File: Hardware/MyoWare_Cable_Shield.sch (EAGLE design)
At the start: 13 parts

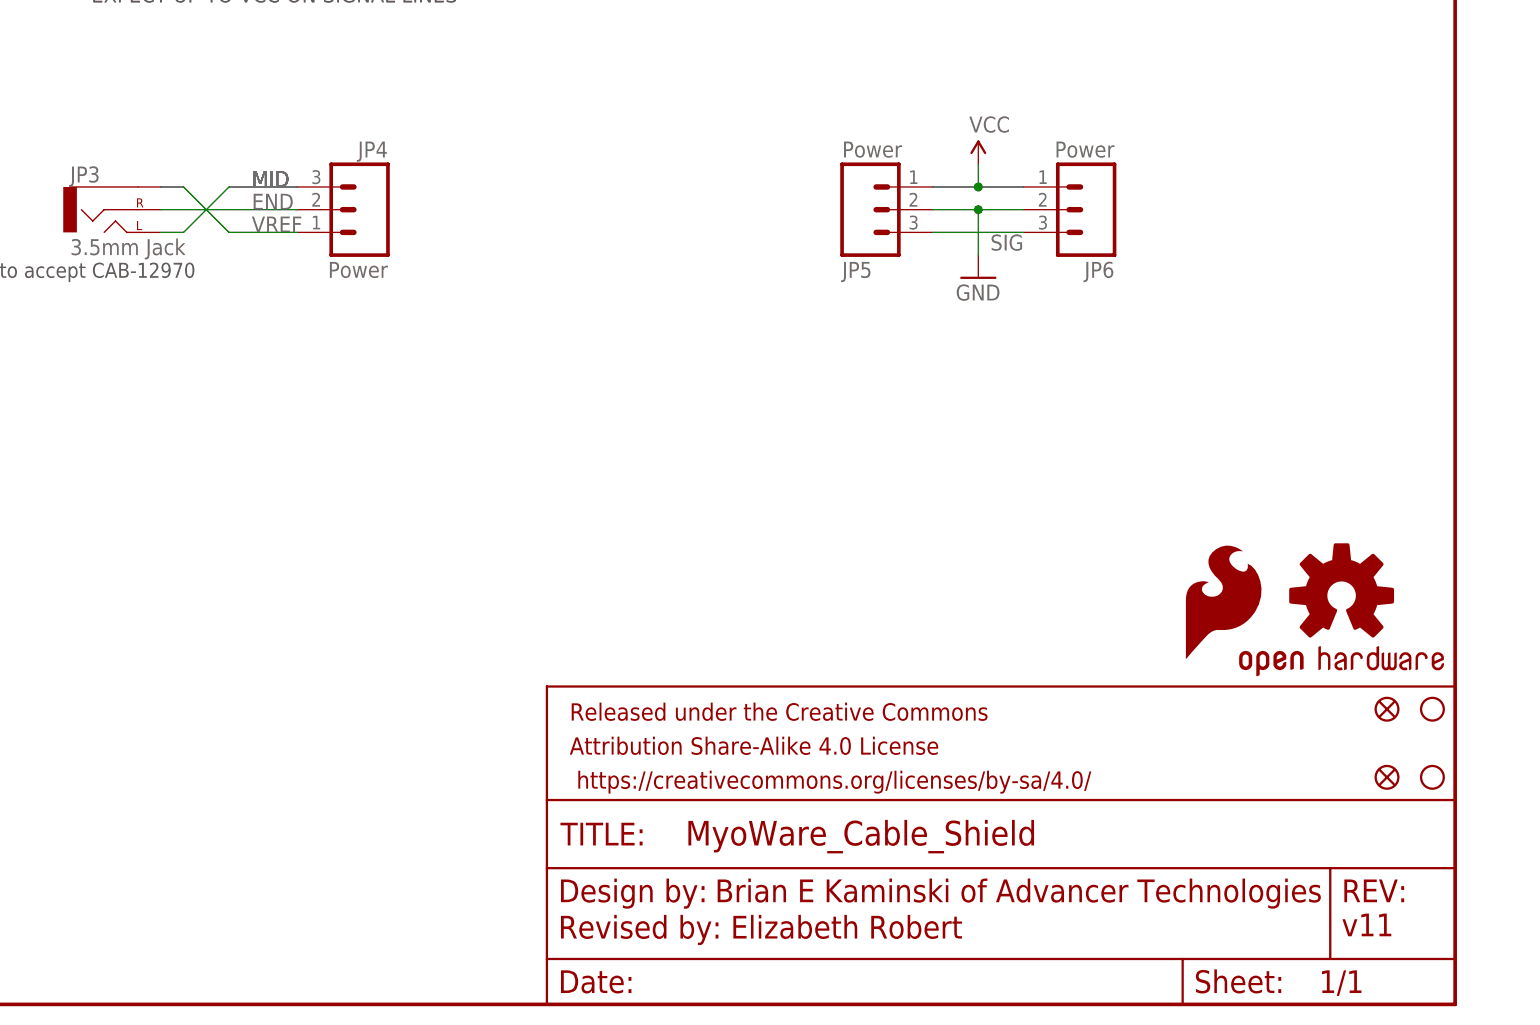
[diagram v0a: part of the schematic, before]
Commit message: Revert "V11"
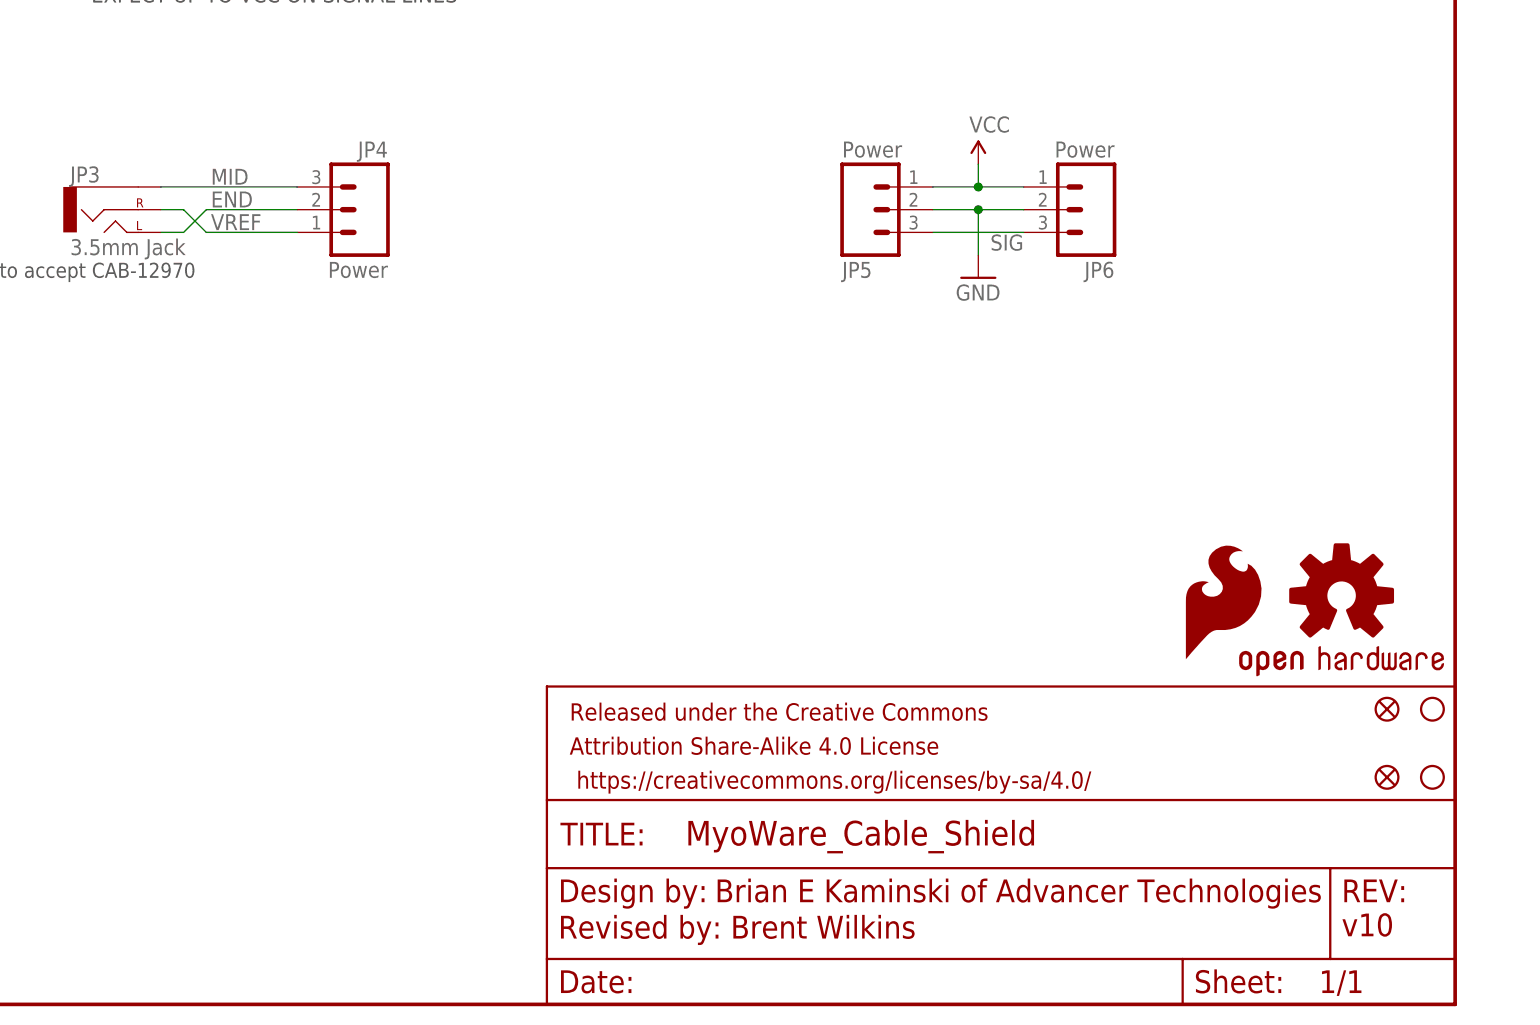
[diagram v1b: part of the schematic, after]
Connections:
- net END: now also JP3.LEFT; no longer JP3.RIGHT
- net MID: now also JP3.SLEEVE; no longer JP3.LEFT
- net VREF: now also JP3.RIGHT; no longer JP3.SLEEVE
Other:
- note added: "Revised by: Brent Wilkins"
- note added: "v10"
- note removed: "Revised by: Elizabeth Robert"
- note removed: "v11"
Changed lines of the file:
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@@
 <?xml version="1.0" encoding="utf-8"?>
 <!DOCTYPE eagle SYSTEM "eagle.dtd">
-<eagle version="7.7.0">
+<eagle version="7.4.0">
 <drawing>
 <settings>
@@
 <plain>
 <text x="166.116" y="11.43" size="2.54" layer="94">Brian E Kaminski of Advancer Technologies</text>
-<text x="148.59" y="7.366" size="2.54" layer="94" ratio="10">Revised by: Elizabeth Robert</text>
-<text x="236.22" y="7.62" size="2.54" layer="94" font="vector">v11</text>
+<text x="148.59" y="7.366" size="2.54" layer="94" ratio="10">Revised by: Brent Wilkins</text>
+<text x="236.22" y="7.62" size="2.54" layer="94" font="vector">v10</text>
 <text x="116.84" y="114.3" size="1.778" layer="97" font="vector" ratio="15" align="center">VCC (+VS) +2.7V to +5.9V
 EXPECT UP TO VCC ON SIGNAL LINES</text>
@@
 </busses>
 <nets>
+<net name="MID" class="0">
+<segment>
+<pinref part="JP4" gate="G$1" pin="3"/>
+<label x="109.728" y="91.694" size="1.778" layer="95"/>
+<wire x1="104.14" y1="91.44" x2="119.38" y2="91.44" width="0.1524" layer="91"/>
+<pinref part="JP3" gate="G$1" pin="SLEEVE"/>
+</segment>
+</net>
+<net name="END" class="0">
+<segment>
+<pinref part="JP4" gate="G$1" pin="2"/>
+<label x="109.728" y="89.154" size="1.778" layer="95"/>
+<wire x1="109.22" y1="88.9" x2="119.38" y2="88.9" width="0.1524" layer="91"/>
+<pinref part="JP3" gate="G$1" pin="LEFT"/>
+<wire x1="104.14" y1="86.36" x2="106.68" y2="86.36" width="0.1524" layer="91"/>
+<wire x1="106.68" y1="86.36" x2="109.22" y2="88.9" width="0.1524" layer="91"/>
+</segment>
+</net>
+<net name="VREF" class="0">
+<segment>
+<pinref part="JP4" gate="G$1" pin="1"/>
+<label x="109.728" y="86.614" size="1.778" layer="95"/>
+<wire x1="109.22" y1="86.36" x2="119.38" y2="86.36" width="0.1524" layer="91"/>
+<pinref part="JP3" gate="G$1" pin="RIGHT"/>
+<wire x1="104.14" y1="88.9" x2="106.68" y2="88.9" width="0.1524" layer="91"/>
+<wire x1="106.68" y1="88.9" x2="109.22" y2="86.36" width="0.1524" layer="91"/>
+</segment>
+</net>
 <net name="SHIELD" class="0">
 <segment>
@@
 </segment>
 </net>
-<net name="MID" class="0">
-<segment>
-<pinref part="JP4" gate="G$1" pin="3"/>
-<wire x1="119.38" y1="91.44" x2="111.76" y2="91.44" width="0.1524" layer="91"/>
-<wire x1="111.76" y1="91.44" x2="106.68" y2="86.36" width="0.1524" layer="91"/>
-<pinref part="JP3" gate="G$1" pin="LEFT"/>
-<wire x1="106.68" y1="86.36" x2="104.14" y2="86.36" width="0.1524" layer="91"/>
-<label x="114.3" y="91.44" size="1.778" layer="95"/>
-<label x="114.3" y="91.44" size="1.778" layer="95"/>
-<label x="114.3" y="91.44" size="1.778" layer="95"/>
-</segment>
-</net>
-<net name="VREF" class="0">
-<segment>
-<pinref part="JP3" gate="G$1" pin="SLEEVE"/>
-<wire x1="104.14" y1="91.44" x2="106.68" y2="91.44" width="0.1524" layer="91"/>
-<wire x1="106.68" y1="91.44" x2="111.76" y2="86.36" width="0.1524" layer="91"/>
-<pinref part="JP4" gate="G$1" pin="1"/>
-<wire x1="111.76" y1="86.36" x2="119.38" y2="86.36" width="0.1524" layer="91"/>
-<label x="114.3" y="86.36" size="1.778" layer="95"/>
-</segment>
-</net>
-<net name="END" class="0">
-<segment>
-<pinref part="JP4" gate="G$1" pin="2"/>
-<pinref part="JP3" gate="G$1" pin="RIGHT"/>
-<wire x1="119.38" y1="88.9" x2="104.14" y2="88.9" width="0.1524" layer="91"/>
-<label x="114.3" y="88.9" size="1.778" layer="95"/>
-</segment>
-</net>
